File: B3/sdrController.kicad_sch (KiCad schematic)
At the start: 5 parts, among them U314 74HC32, U316 74HC00, U317 74HC74, U318 74HC08, U319 74HC32

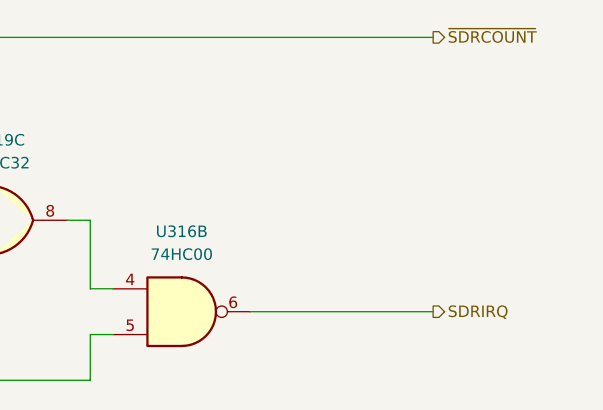
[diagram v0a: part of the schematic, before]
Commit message: .
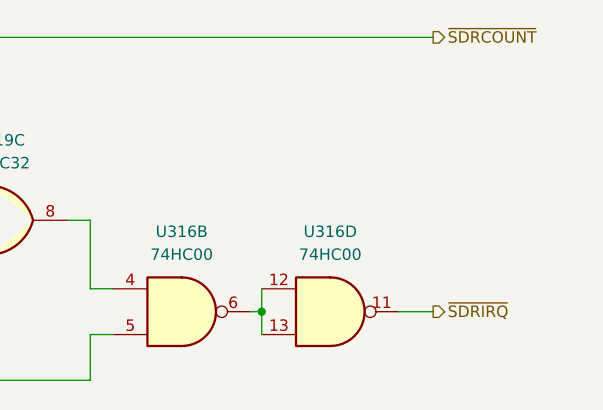
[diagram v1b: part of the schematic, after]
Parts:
- added unit 4 of U316
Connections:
- net SDRIRQ: no longer names the net of U316.6
- net SDRIRQ: now also U316.12, U316.13
- new net ~{SDRIRQ}: U316.11
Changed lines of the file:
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@@
   (junction (at 127 68.58) (diameter 0) (color 0 0 0 0)
+  )
+  (junction (at 224.79 152.4) (diameter 0) (color 0 0 0 0)
   )
   (junction (at 137.16 152.4) (diameter 0) (color 0 0 0 0)
@@
     (stroke (width 0) (type default) (color 0 0 0 0))
   )
-  (wire (pts (xy 223.52 152.4) (xy 243.84 152.4))
-    (stroke (width 0) (type default) (color 0 0 0 0))
-  )
   (wire (pts (xy 182.88 109.22) (xy 185.42 109.22))
     (stroke (width 0) (type default) (color 0 0 0 0))
@@
     (stroke (width 0) (type default) (color 0 0 0 0))
   )
+  (wire (pts (xy 224.79 152.4) (xy 224.79 154.94))
+    (stroke (width 0) (type default) (color 0 0 0 0))
+  )
   (wire (pts (xy 91.44 116.84) (xy 114.3 116.84))
     (stroke (width 0) (type default) (color 0 0 0 0))
@@
     (stroke (width 0) (type default) (color 0 0 0 0))
   )
+  (wire (pts (xy 240.03 152.4) (xy 243.84 152.4))
+    (stroke (width 0) (type default) (color 0 0 0 0))
+  )
+  (wire (pts (xy 224.79 152.4) (xy 224.79 149.86))
+    (stroke (width 0) (type default) (color 0 0 0 0))
+  )
   (wire (pts (xy 116.84 40.64) (xy 116.84 38.1))
     (stroke (width 0) (type default) (color 0 0 0 0))
@@
   )
   (wire (pts (xy 83.82 71.12) (xy 106.68 71.12))
+    (stroke (width 0) (type default) (color 0 0 0 0))
+  )
+  (wire (pts (xy 223.52 152.4) (xy 224.79 152.4))
     (stroke (width 0) (type default) (color 0 0 0 0))
   )
@@
     (effects (font (size 1.27 1.27)) (justify right))
   )
-  (hierarchical_label "SDRIRQ" (shape output) (at 243.84 152.4 0)
+  (hierarchical_label "~{SDRIRQ}" (shape output) (at 243.84 152.4 0)
     (effects (font (size 1.27 1.27)) (justify left))
   )
@@
     (effects (font (size 1.27 1.27)) (justify right))
   )
+  (symbol (lib_id "74xx:74HC00") (at 232.41 152.4 0) (unit 4)
+    (in_bom yes) (on_board yes) (fields_autoplaced)
+    (property "Reference" "U316" (id 0) (at 232.41 143.51 0))
+    (property "Value" "74HC00" (id 1) (at 232.41 146.05 0))
+    (property "Footprint" "Package_SO:SO-14_3.9x8.65mm_P1.27mm" (id 2) (at 232.41 152.4 0)
+      (effects (font (size 1.27 1.27)) hide)
+    )
+    (property "Datasheet" "http://www.ti.com/lit/gpn/sn74hc00" (id 3) (at 232.41 152.4 0)
+      (effects (font (size 1.27 1.27)) hide)
+    )
+    (pin "1")
+    (pin "2")
+    (pin "3")
+    (pin "4")
+    (pin "5")
+    (pin "6")
+    (pin "10")
+    (pin "8")
+    (pin "9")
+    (pin "11")
+    (pin "12")
+    (pin "13")
+    (pin "14")
+    (pin "7")
+  )
   (symbol (lib_id "Custom 74xx:74HC08") (at 175.26 71.12 0) (unit 4)
